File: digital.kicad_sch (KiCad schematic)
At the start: 33 parts

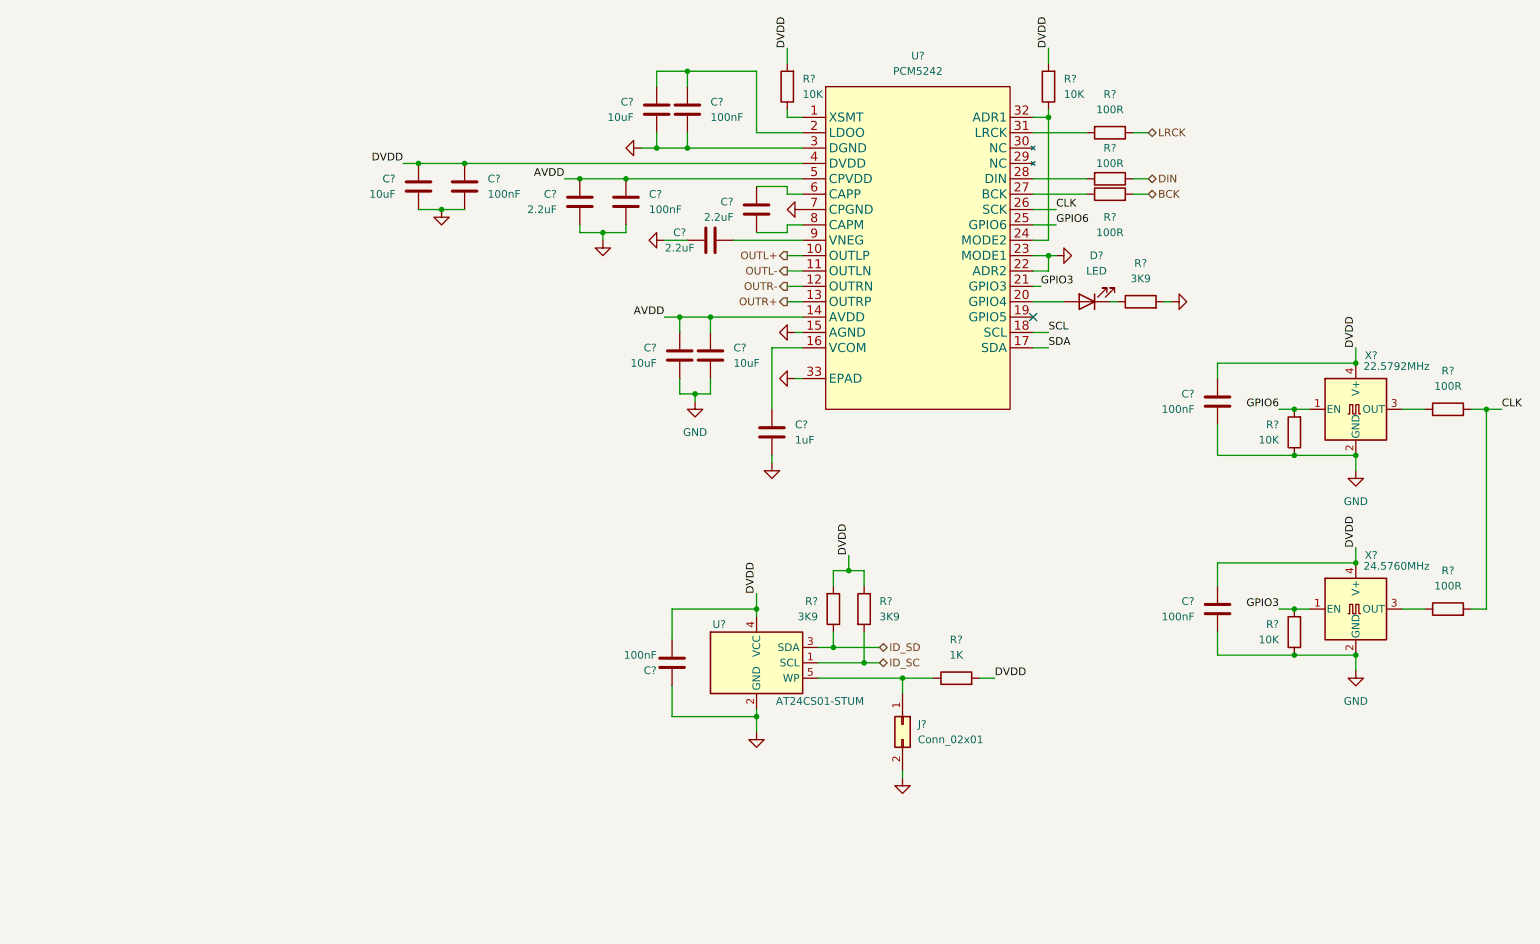
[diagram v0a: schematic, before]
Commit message: WIP
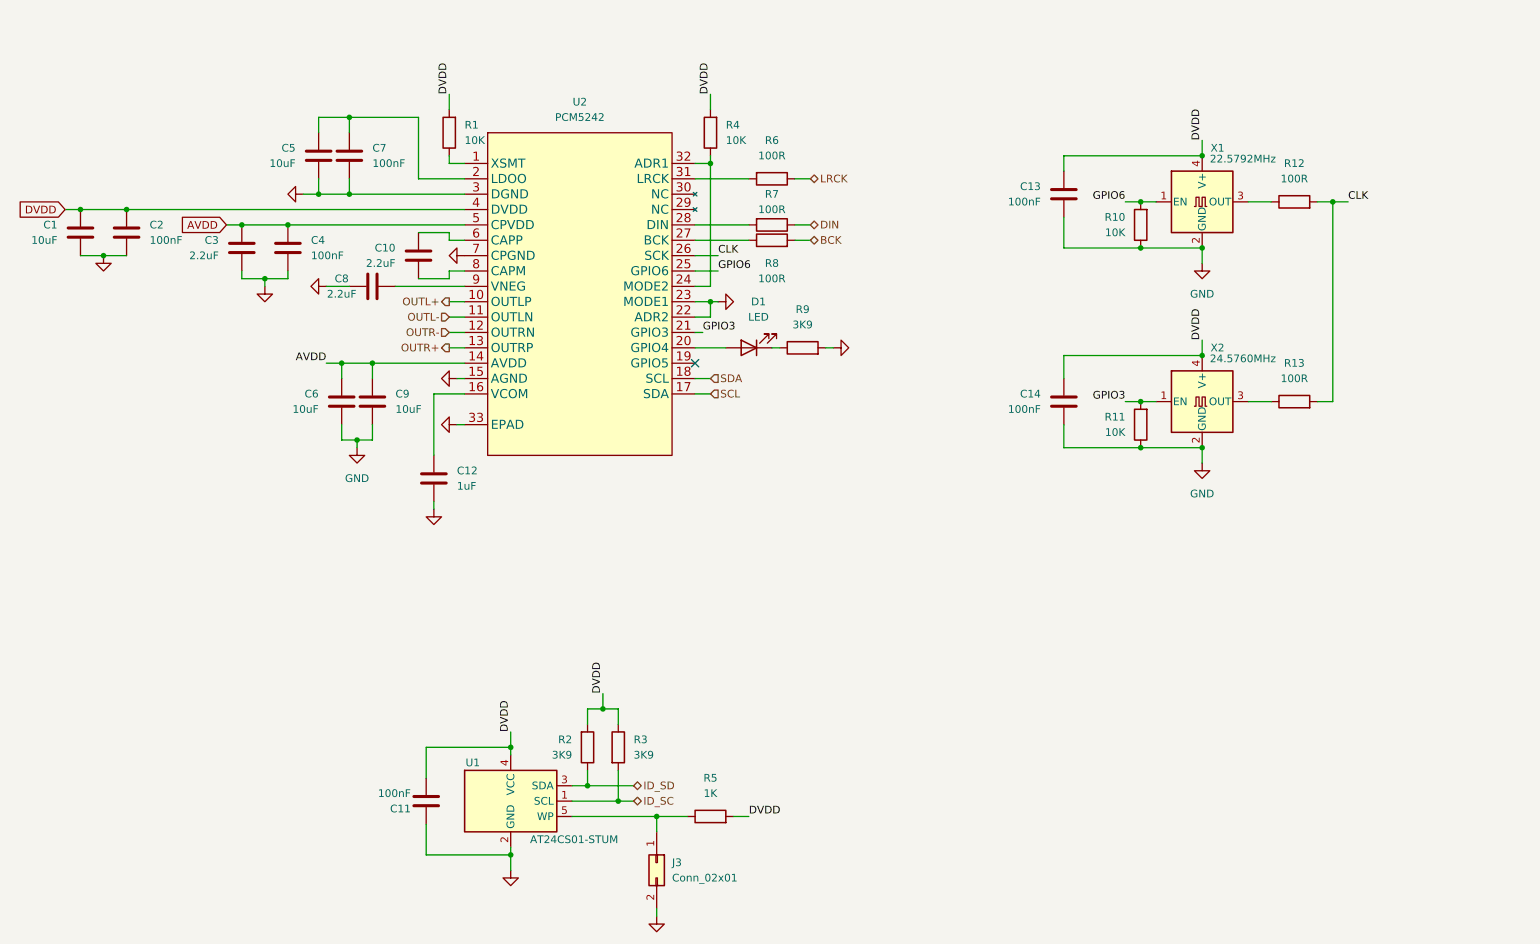
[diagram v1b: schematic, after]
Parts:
- gave numbers to parts that had none: 33
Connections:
- net SCL: now also U2.17 (SDA); no longer U2.18 (SCL)
- net SDA: now also U2.18 (SCL); no longer U2.17 (SDA)
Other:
- moved on the sheet: C1, C10, C11, C12, C13, C14, C2, C3, C4, C5, C6, C7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
